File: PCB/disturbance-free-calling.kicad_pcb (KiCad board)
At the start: 2 copper layers, 74.5 x 20 mm, 22 parts, among them U1 MOUDLE-SEEEDUINO-XIAO-ESP32C3

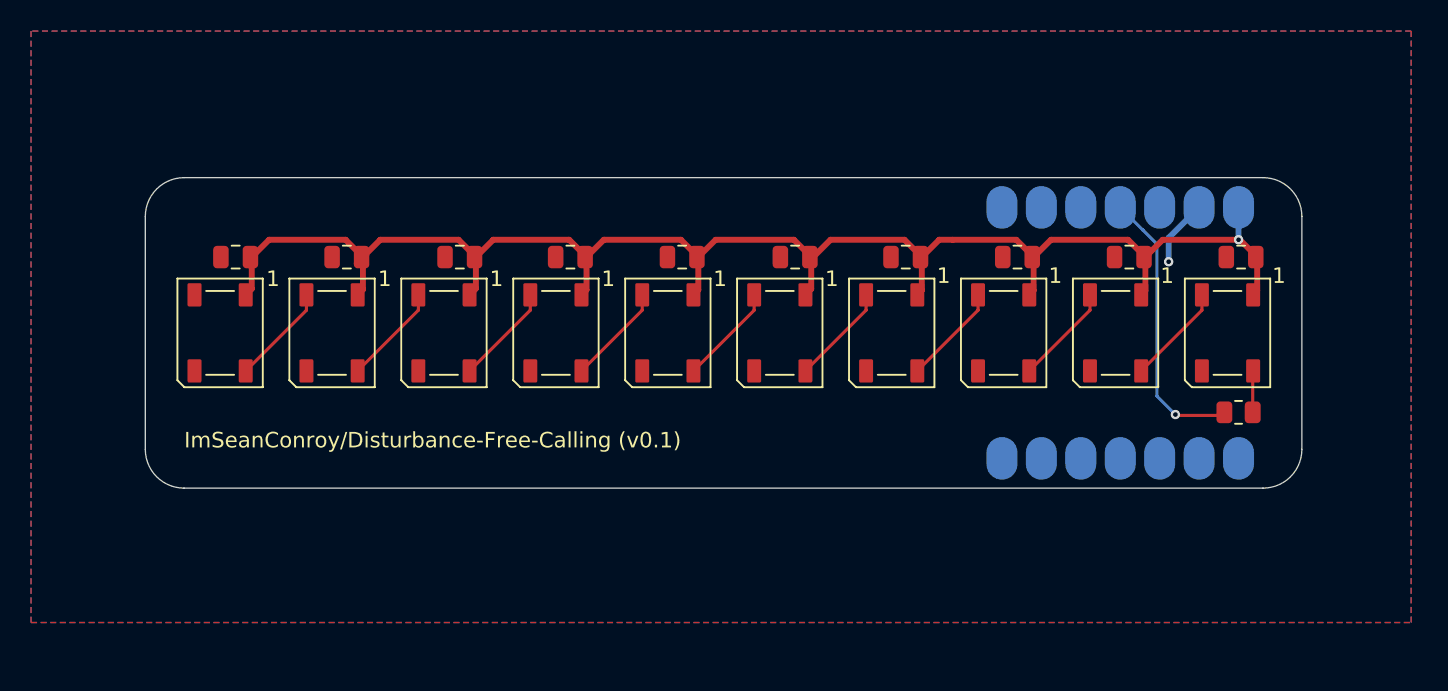
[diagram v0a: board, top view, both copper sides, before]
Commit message: Rearrange layout
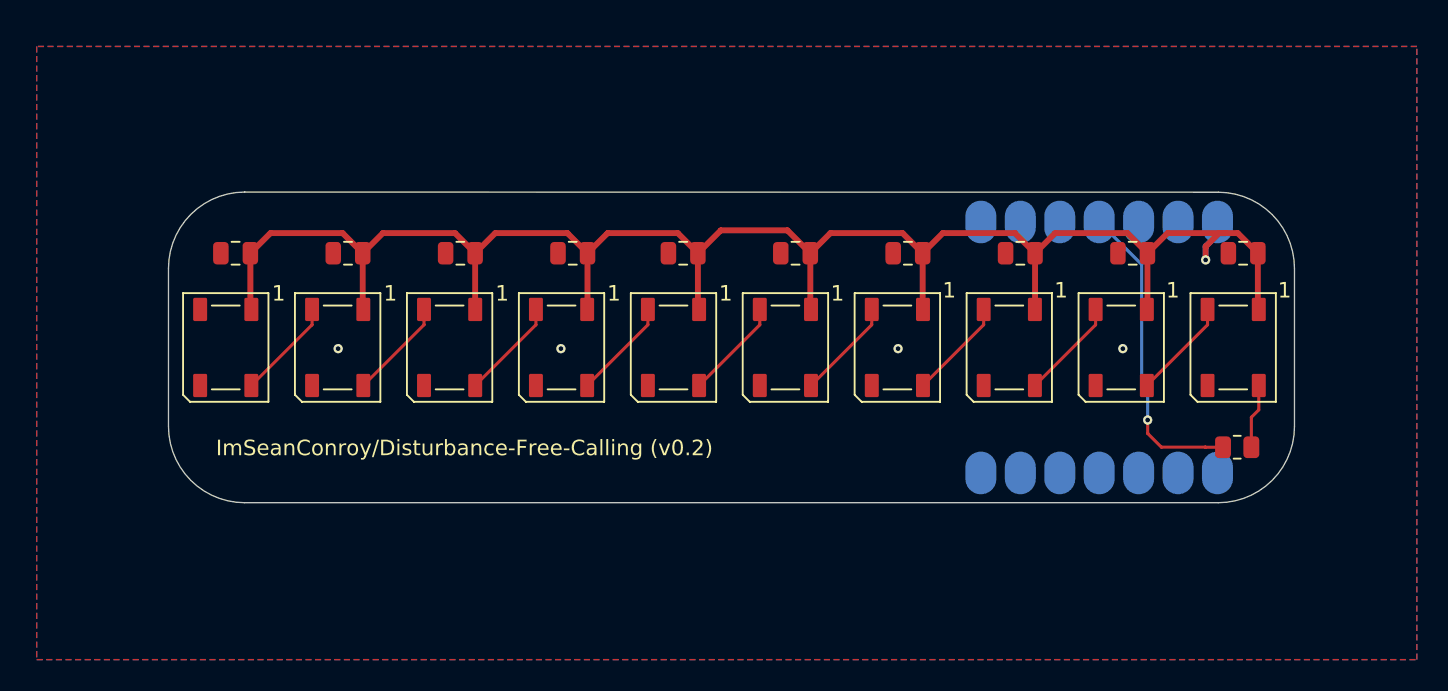
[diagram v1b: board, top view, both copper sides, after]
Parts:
- U1: footprint xiao ESP32C3_PCB:MOUDLE14P-SMD-2.54-21X17.8MM -> MOUDLE-SEEEDUINO-XIAO-ESP32C3:MOUDLE14P-SMD-2.54-21X17.8MM
- moved R1 2.25 mm to (135.9, 70.0)
- moved U1 1.65 mm to (116.5, 72.5)
- moved D1 1.01 mm to (135.6, 63.5)
- moved D10 1.01 mm to (70.7, 63.5)
- moved D2 1.01 mm to (128.4, 63.5)
- moved D3 1.01 mm to (121.2, 63.5)
- moved D4 1.01 mm to (114.0, 63.5)
- moved D5 1.01 mm to (106.8, 63.5)
- moved D6 1.01 mm to (99.6, 63.5)
- moved D7 1.01 mm to (92.4, 63.5)
- moved D8 1.01 mm to (85.2, 63.5)
- moved D9 1.01 mm to (77.9, 63.5)
- moved C2 0.33 mm to (129.2, 57.5)
- moved C3 0.31 mm to (121.9, 57.5)
- moved C7 0.29 mm to (93.1, 57.5)
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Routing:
- net +5V: track 101.9 -> 116.3 mm
- net GND: track 5.97 -> 0.00 mm, vias 1 -> 4
- net Net-(U1-PA6_A10_D10_MOSI): track 18.0 -> 20.1 mm
- net DATA: track 2.88 -> 4.18 mm
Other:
- board size 74.5 x 20 mm -> 72.5 x 20 mm
- board text added: "ImSeanConroy/Disturbance-Free-Calling (v0.2)"
- board text removed: "ImSeanConroy/Disturbance-Free-Calling (v0.1)"
